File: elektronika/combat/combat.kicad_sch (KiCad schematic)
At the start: 35 parts, among them J1 odbiornik, J2 naped_prawy, J3 naped_lewy, J4 buzzer, J5 wyjscie do silnika +-, J6 programator od adama wasa, J7 zasilanie xt30, J8 Conn_01x01_Pin, J800 USB_C_Receptacle_USB2.0_16P, U1 ESP32-S3-WROOM-1, U2 kontroler_bldc, U3 AMS1117, U4 przetwornica

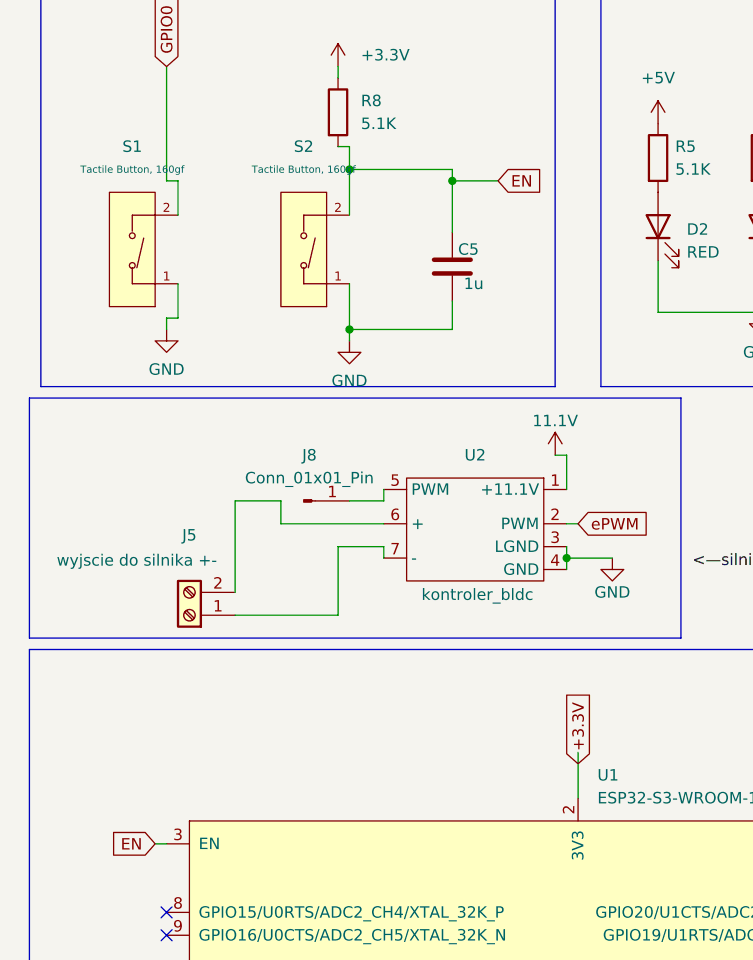
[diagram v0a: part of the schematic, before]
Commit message: dostosowano reguly do jlcpcb
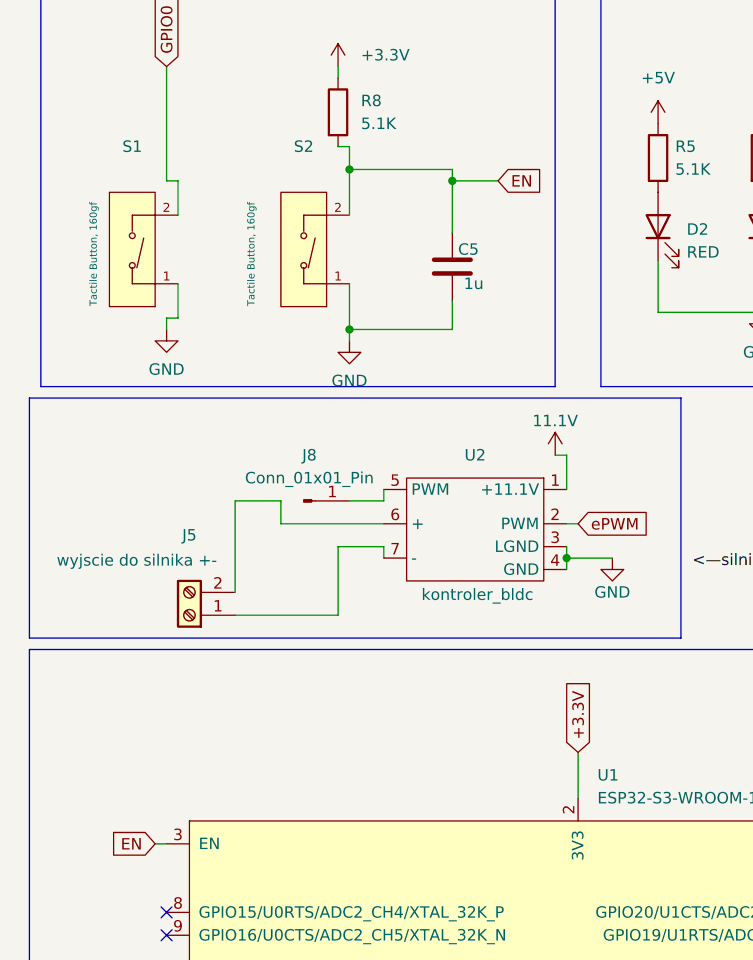
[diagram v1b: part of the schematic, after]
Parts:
- C1: footprint Capacitor_SMD:C_0805_2012Metric_Pad1.18x1.45mm_HandSolder -> Capacitor_SMD:C_0603_1608Metric_Pad1.08x0.95mm_HandSolder
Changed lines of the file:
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@@
 	(wire
 		(pts
+			(xy 74.93 109.22) (xy 74.93 104.14)
+		)
+		(stroke
+			(width 0)
+			(type default)
+		)
+	)
+	(wire
+		(pts
 			(xy 246.38 138.43) (xy 250.19 138.43)
 		)
@@
 	(wire
 		(pts
-			(xy 74.93 104.14) (xy 74.93 109.22)
-		)
-		(stroke
-			(width 0)
-			(type default)
-		)
-	)
-	(wire
-		(pts
 			(xy 60.96 40.64) (xy 60.96 46.355)
 		)
@@
 	(global_label "+3.3V"
 		(shape input)
-		(at 74.93 105.41 90)
+		(at 74.93 104.14 90)
 		(fields_autoplaced yes)
 		(effects
@@
 		)
 		(property "Intersheetrefs" "${INTERSHEET_REFS}"
-			(at 74.93 96.74 90)
+			(at 74.93 95.47 90)
 			(hide yes)
 			(show_name no)
@@
 		(in_pos_files yes)
 		(dnp no)
-		(fields_autoplaced yes)
 		(property "Reference" "S1"
 			(at 25.4 36.83 0)
@@
 		)
 		(property "Value" "Tactile Button, 160gf"
-			(at 25.4 39.37 0)
+			(at 21.082 48.768 90)
 			(show_name no)
 			(do_not_autoplace no)
@@
 		(in_pos_files yes)
 		(dnp no)
-		(fields_autoplaced yes)
 		(property "Reference" "S2"
 			(at 44.45 36.83 0)
@@
 		)
 		(property "Value" "Tactile Button, 160gf"
-			(at 44.45 39.37 0)
+			(at 38.608 48.768 90)
 			(show_name no)
 			(do_not_autoplace no)
@@
 			)
 		)
-		(property "Footprint" "Capacitor_SMD:C_0805_2012Metric_Pad1.18x1.45mm_HandSolder"
+		(property "Footprint" "Capacitor_SMD:C_0603_1608Metric_Pad1.08x0.95mm_HandSolder"
 			(at 211.7852 63.5 0)
 			(hide yes)
